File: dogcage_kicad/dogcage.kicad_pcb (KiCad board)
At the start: 2 copper layers, 76.2 x 49.5 mm, 18 parts, among them CON1 BARREL_JACK, M1 XBEE, P1 Door Sensor, P2 Servo, P3 CONN_01X10, P4 CONN_01X10, P5 CONN_01X14, P6 CONN_01X05, P7 CONN_01X14, Q1 TIP120, SW1 SW_PUSH, U1 LD1117S33TR, U2 TEENSYLC

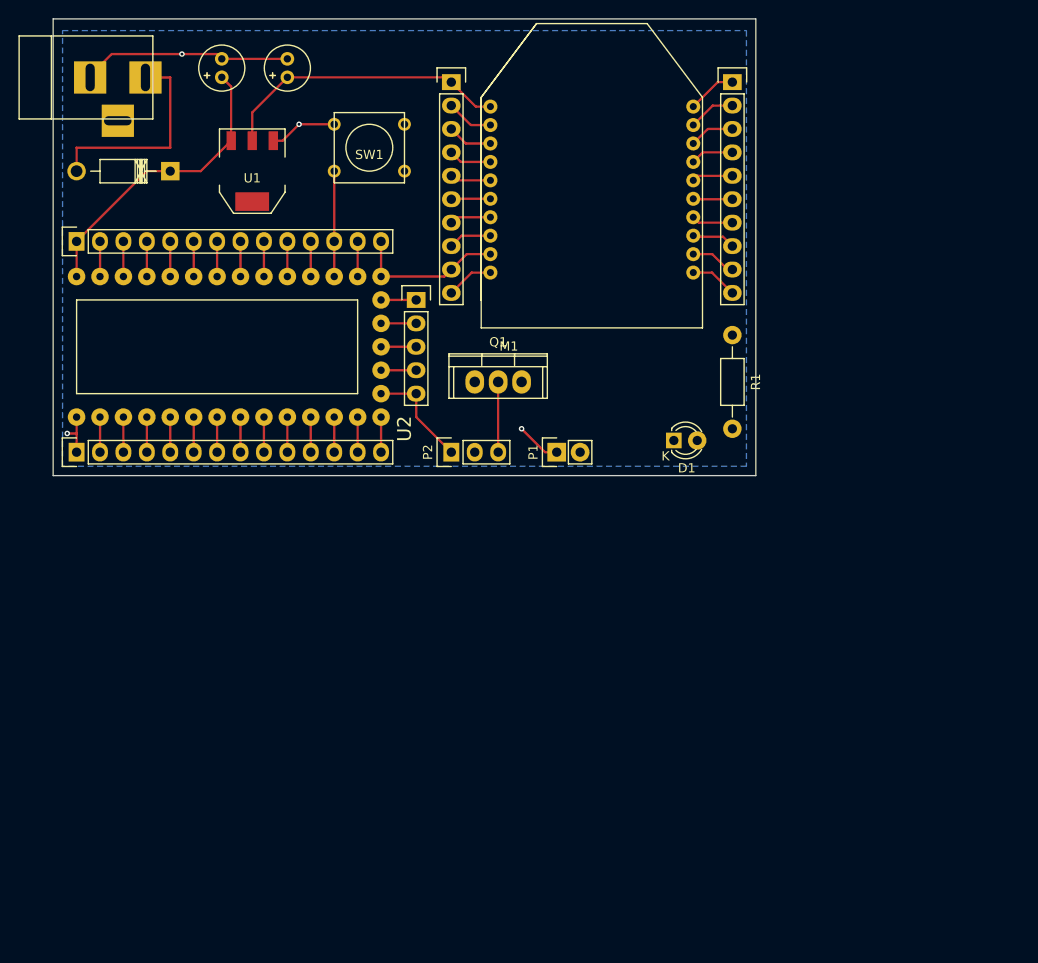
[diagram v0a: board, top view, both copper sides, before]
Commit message: Routing complete
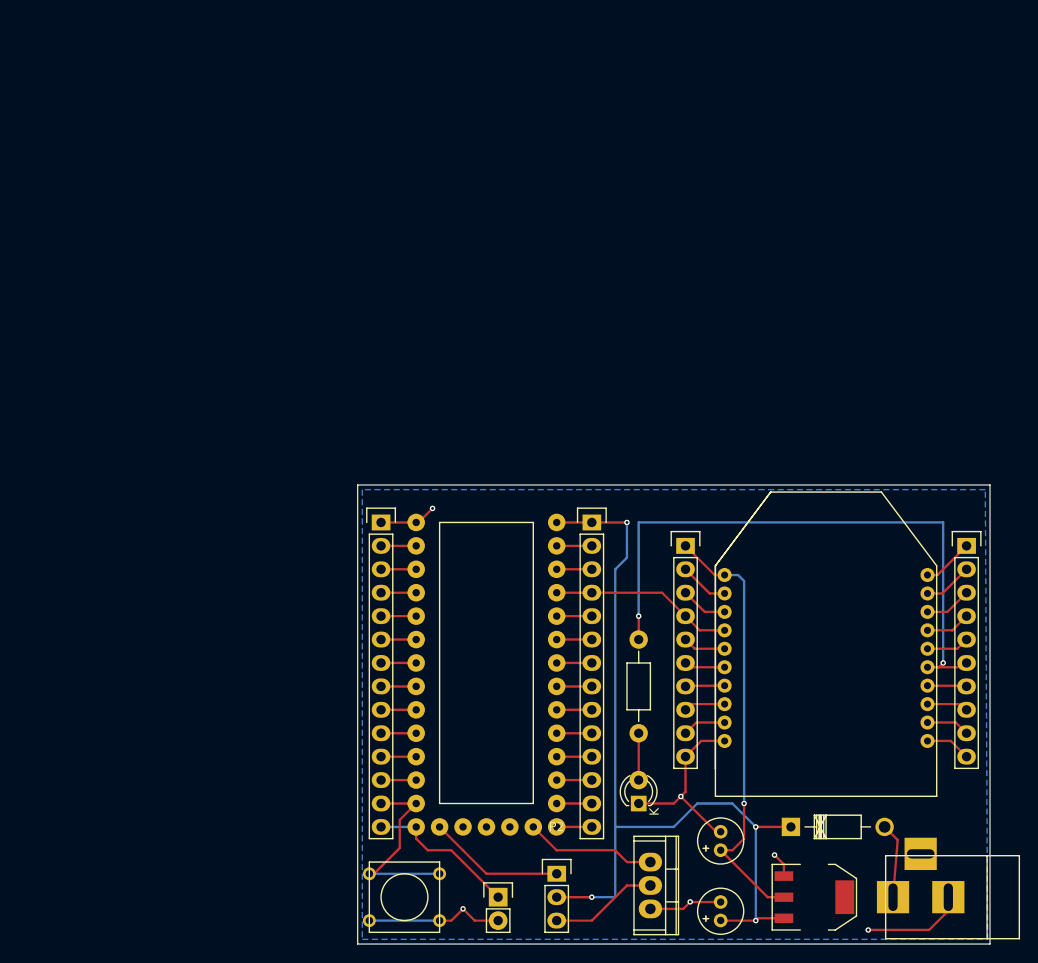
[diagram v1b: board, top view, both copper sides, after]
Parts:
- removed P6: CONN_01X05, Pin_Headers:Pin_Header_Straight_1x05
- CON1: value BARREL_JACK -> 5V
- D1: value Assoc LED -> Assoc
- P1: value Door Sensor -> Door
- moved CON1 129.0 mm to (193.8, 170.2), turned to 180 degrees
- moved C1 106.2 mm to (168.9, 172.7)
- moved U1 99.6 mm to (179.1, 170.2), turned to 270 degrees
- moved D2 97.9 mm to (176.5, 162.6), turned to 0 degrees
- moved C2 96.1 mm to (168.9, 165.1)
- moved SW1 81.4 mm to (134.6, 170.2), turned to 0 degrees
- moved P7 63.7 mm to (154.9, 129.5), turned to 0 degrees
- moved Q1 57.1 mm to (161.3, 168.9), turned to 270 degrees
- moved M1 56.8 mm to (180.3, 142.2)
- moved P3 56.3 mm to (165.1, 132.1)
- moved P4 56.3 mm to (195.6, 132.1)
- moved P1 48.7 mm to (144.8, 170.2), turned to 0 degrees
- moved P2 47.1 mm to (151.1, 167.6), turned to 0 degrees
- moved D1 39.6 mm to (160.0, 160.0), turned to 90 degrees
- moved U2 37.0 mm to (135.9, 132.1), turned to 270 degrees
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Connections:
- M1 pad 4: Net-(M1-Pad4) -> /XBEE_CTL
- M1 pad 9: /XBEE_CTL -> Net-(M1-Pad9)
- P3 pad 4: Net-(M1-Pad4) -> /XBEE_CTL
- P3 pad 9: /XBEE_CTL -> Net-(M1-Pad9)
- P5 pad 12: Net-(P1-Pad1) -> Net-(P5-Pad12)
- P5 pad 14: Net-(P5-Pad14) -> Net-(P1-Pad1)
- P7 pad 14: /XBEE_CTL -> Net-(P7-Pad14)
- P7 pad 4: Net-(P7-Pad4) -> /XBEE_CTL
- Q1 pad 1: Net-(P5-Pad14) -> Net-(Q1-Pad1)
- SW1 pad 1: Net-(P7-Pad12) -> Net-(P5-Pad13)
- U2 pad 12: Net-(P1-Pad1) -> Net-(P5-Pad12)
- U2 pad 14: Net-(P5-Pad14) -> Net-(P1-Pad1)
- U2 pad 19: Net-(P6-Pad1) -> Net-(Q1-Pad1)
- U2 pad 20: /XBEE_CTL -> Net-(P7-Pad14)
- U2 pad 30: Net-(P7-Pad4) -> /XBEE_CTL
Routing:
- net Net-(M1-Pad15): track 4.26 -> 67.3 mm, vias 0 -> 2
- net +5V: track 32.4 -> 93.8 mm, vias 0 -> 4
- net GND: track 40.1 -> 63.2 mm, vias 3 -> 6
- net Net-(P5-Pad13): track 3.81 -> 21.5 mm
- net +3V3: track 31.8 -> 47.9 mm, vias 0 -> 1
- net Net-(CON1-Pad1): track 23.0 -> 8.23 mm
- net Net-(Q1-Pad1): track 0.00 -> 14.3 mm
- net Net-(P1-Pad1): track 8.67 -> 16.6 mm, vias 1 -> 0
- net Net-(P7-Pad12): track 11.4 -> 3.81 mm
- net Net-(D1-Pad2): track 0.00 -> 5.08 mm
- net Net-(M1-Pad9): track 0.00 -> 4.72 mm
- net Net-(M1-Pad4): track 4.67 -> 0.00 mm
- net Net-(P2-Pad3): track 7.62 -> 11.7 mm
- net Net-(P7-Pad4): track 3.81 -> 0.00 mm
- net Net-(P7-Pad14): track 0.00 -> 3.81 mm
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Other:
- board size 76.2 x 49.5 mm -> 68.6 x 49.8 mm
